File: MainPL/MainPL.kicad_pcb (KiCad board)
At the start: 2 copper layers, 113 x 155.6 mm, 37 parts, among them J1 Conn_01x06_Female, J10 Conn_01x06_Female, J11 Conn_01x06_Female, J12 Conn_01x06_Female, J13 Conn_01x06_Female, J14 Conn_01x06_Female, J15 Conn_01x01_Male, J16 Conn_01x04_Male, J2 USB_B, J3 Conn_01x06_Female, J4 Conn_01x06_Female, J5 Conn_01x06_Female, J6 Conn_01x06_Female, J7 Conn_01x09_Male, J8 Conn_01x06_Female, J9 Conn_01x06_Female, SW1 SW_Push_Dual, U1 74LS32, U2 ATmega328P-PU, U3 MCP23017_SP, U5 MCP23017_SP, U6 74LS373, U7 MCP23017_SP, U8 MC74HC589A, U9 74LVC2G04, Y1 Crystal_GND2

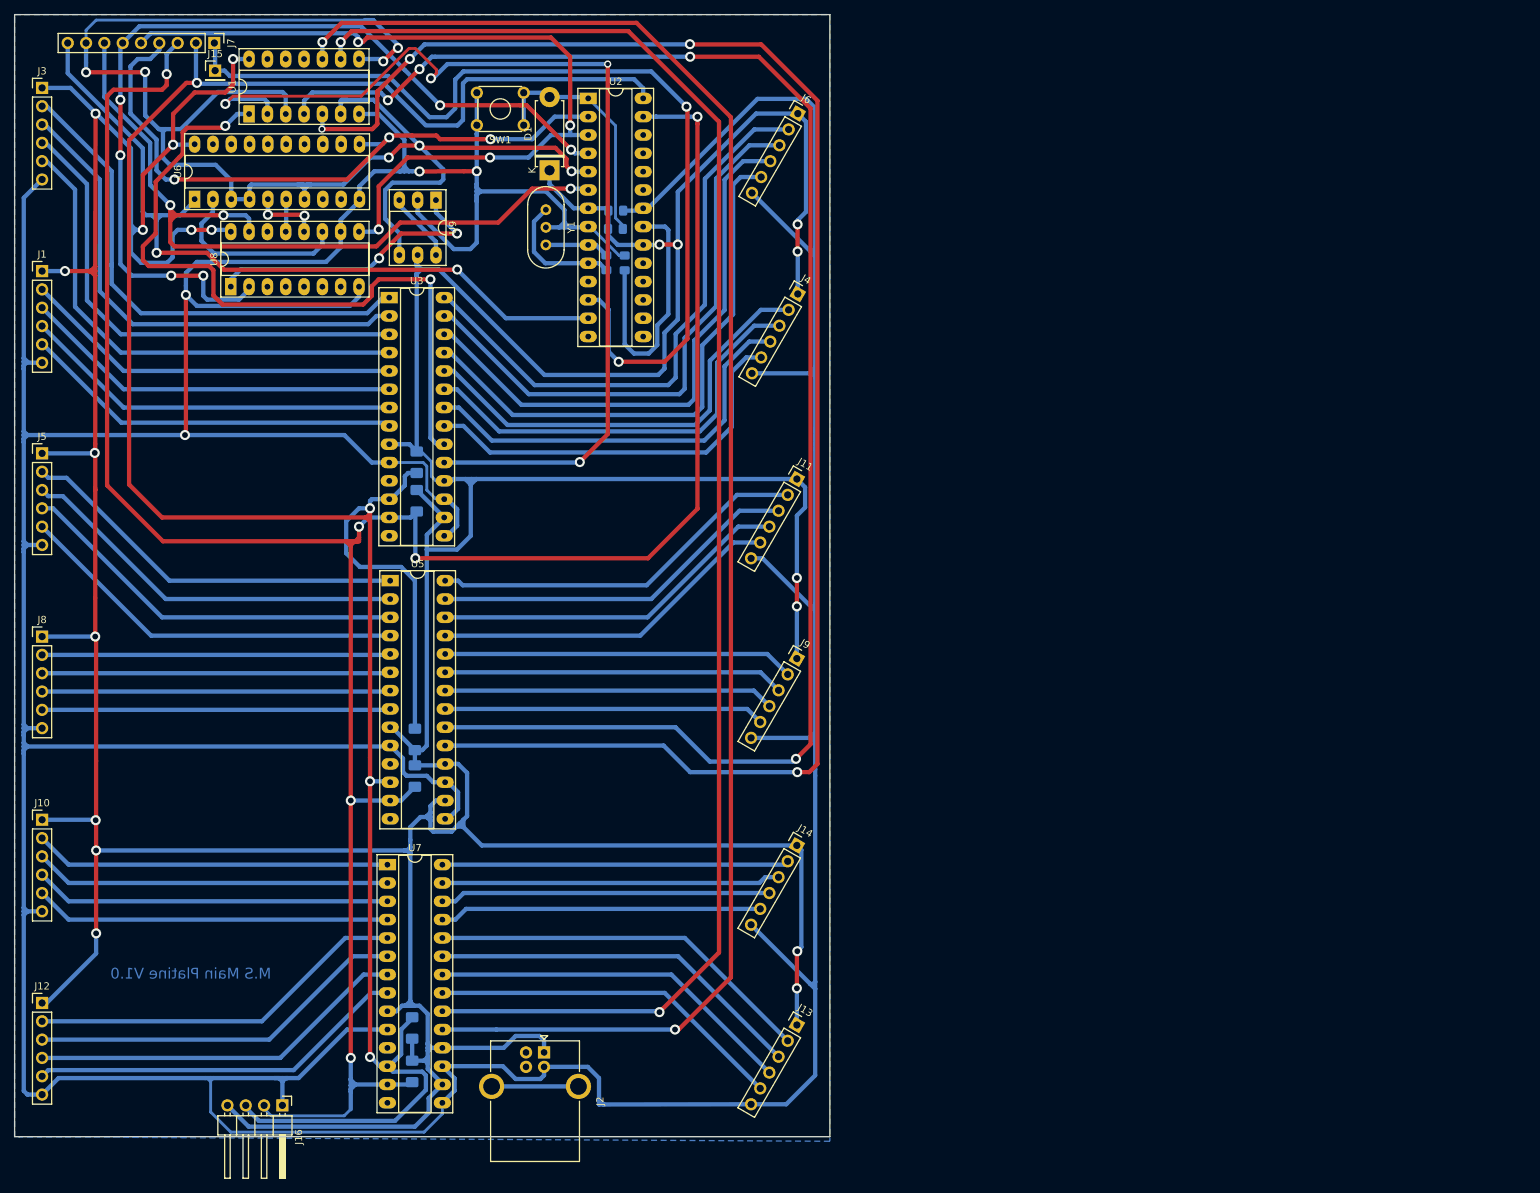
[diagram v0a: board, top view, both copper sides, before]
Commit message: Add files via upload
V.2 von Parkplatz mit neuen Maßen
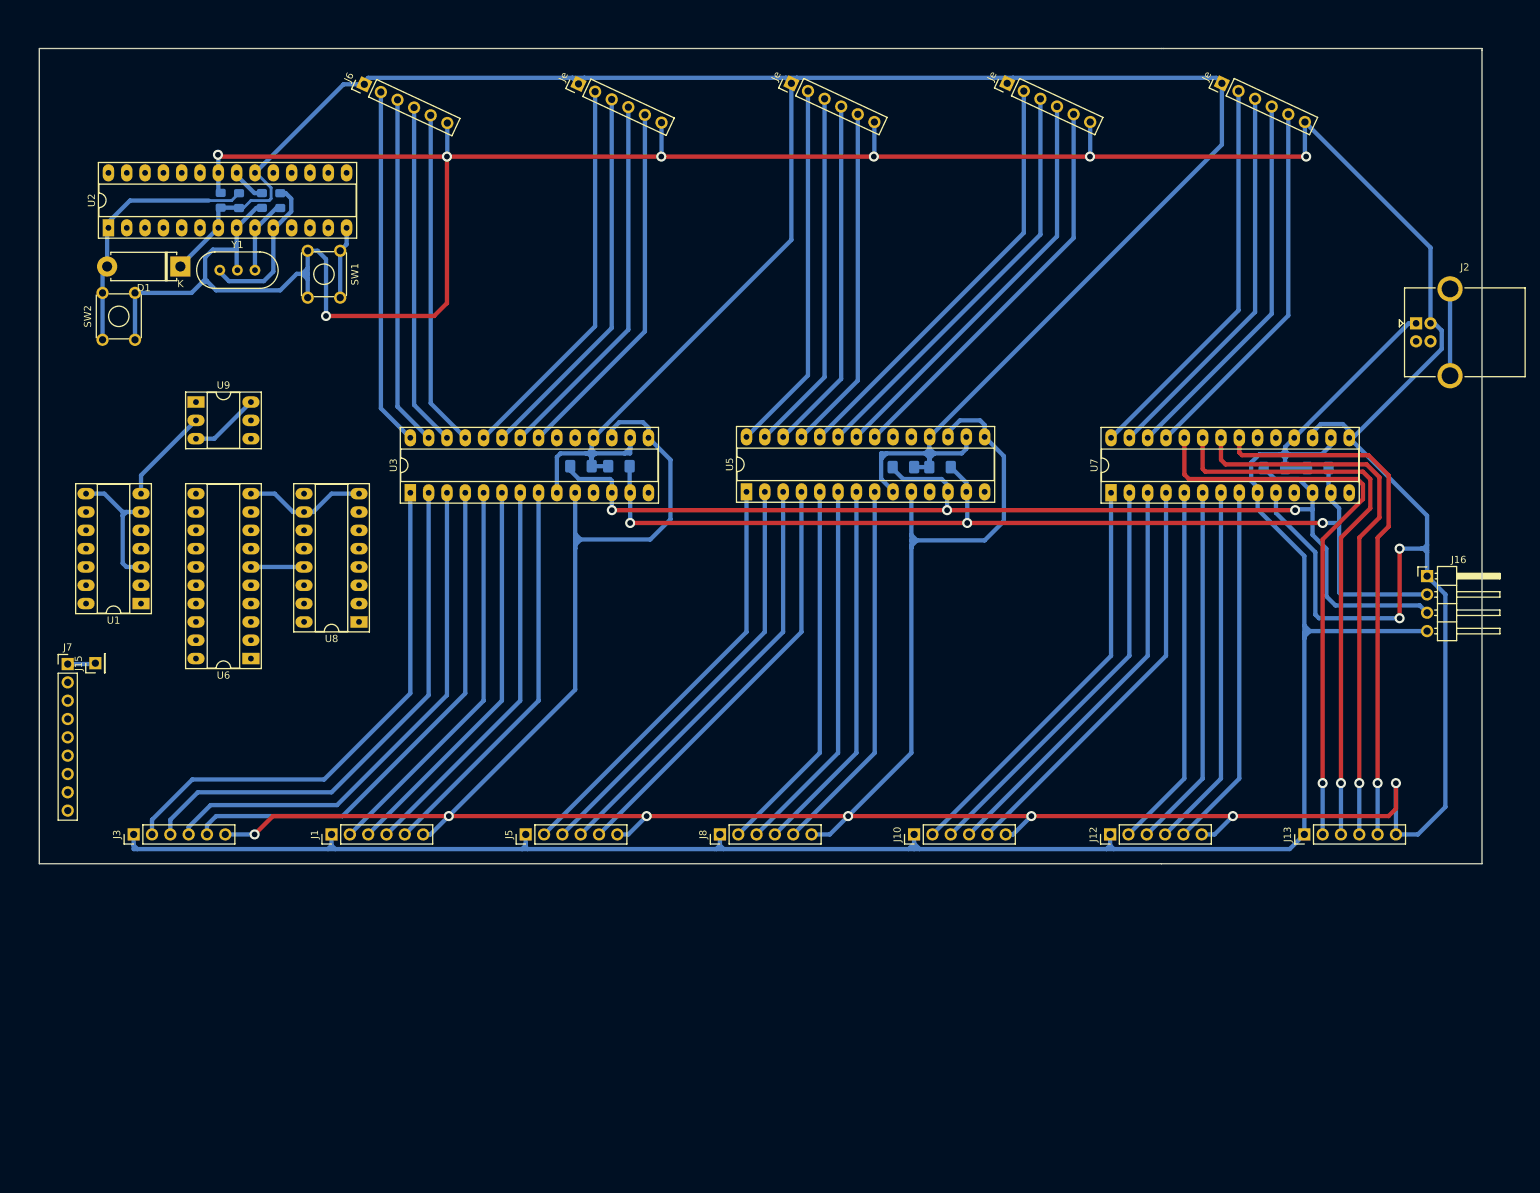
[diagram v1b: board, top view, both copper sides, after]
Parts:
- removed J14, J4, J9: Conn_01x06_Female, Connector_PinHeader_2.54mm:PinHeader_1x06_P2.54mm_Vertical
- added Je: Conn_01x06_Female, Connector_PinHeader_2.54mm:PinHeader_1x06_P2.54mm_Vertical, F.Cu at (122.6, 35.6)
- added Je: Conn_01x06_Female, Connector_PinHeader_2.54mm:PinHeader_1x06_P2.54mm_Vertical, F.Cu at (182.1, 35.6)
- added Je: Conn_01x06_Female, Connector_PinHeader_2.54mm:PinHeader_1x06_P2.54mm_Vertical, F.Cu at (211.8, 35.6)
- added SW2: SW_Push_MS, Button_Switch_THT:SW_TH_Tactile_Omron_B3F-10xx, F.Cu at (56.6, 71.1)
- SW1: value SW_Push_Dual -> SW_Push_MS
- moved J16 174.8 mm to (240.3, 103.9), turned to 0 degrees
- moved J2 157.6 mm to (238.8, 68.8), turned to 0 degrees
- moved R6 150.9 mm to (225.1, 88.9), turned to 0 degrees
- moved J12 149.9 mm to (196.3, 139.7), turned to 90 degrees
- moved R8 142.5 mm to (219.1, 88.9), turned to 0 degrees
- moved J10 120.9 mm to (169.2, 139.7), turned to 90 degrees
- moved U7 112.8 mm to (196.5, 92.3), turned to 90 degrees
- moved J3 104.3 mm to (61.0, 139.7), turned to 90 degrees
- moved J8 97.9 mm to (142.2, 139.7), turned to 90 degrees
- moved J7 88.5 mm to (51.8, 116.1), turned to 0 degrees
- moved J1 87.8 mm to (88.4, 139.7), turned to 90 degrees
- moved J5 85.4 mm to (115.3, 139.7), turned to 90 degrees
- moved R3 84.5 mm to (172.8, 88.8), turned to 0 degrees
- moved J15 83.8 mm to (55.6, 116.0), turned to 90 degrees
- moved R4 77.5 mm to (167.7, 88.8), turned to 0 degrees
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- renumbered J11 to Je
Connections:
- net /INTB_2 renamed Net-(U1-Pad5)
- SW1 pad 1: Net-(D1-Pad2) -> Net-(SW1-Pad1)
- SW1 pad 2: GND -> Net-(SW1-Pad1)
- SW1 pad 3: Net-(D1-Pad2) -> GND
- U2 pad 14: Net-(U2-Pad14) -> Net-(SW1-Pad1)
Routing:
- net Net-(U1-Pad10): track 227.8 -> 0.00 mm, vias 2 -> 0
- net Net-(U1-Pad5): track 227.4 -> 0.00 mm, vias 4 -> 0
- net Net-(U1-Pad4): track 220.3 -> 0.00 mm, vias 4 -> 0
- net Net-(U1-Pad9): track 217.7 -> 0.00 mm, vias 2 -> 0
- net /SDA: track 345.7 -> 145.1 mm, vias 6 -> 3
- net /INTArduino: track 218.0 -> 19.3 mm, vias 7 -> 0
- net /SCL: track 350.5 -> 158.8 mm, vias 4 -> 3
- net +5V: track 821.1 -> 661.1 mm, vias 20 -> 0
- net Net-(U1-Pad2): track 144.1 -> 0.00 mm, vias 4 -> 0
- net Servo: track 133.2 -> 3.88 mm, vias 2 -> 0
- net /CLK: track 126.1 -> 0.00 mm, vias 6 -> 0
- net /Qh: track 114.1 -> 0.00 mm, vias 4 -> 0
- net /CLK_INH: track 108.7 -> 0.00 mm, vias 3 -> 0
- net /OE: track 106.8 -> 0.00 mm, vias 2 -> 0
- net Net-(U1-Pad1): track 102.1 -> 0.00 mm, vias 2 -> 0
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- removed copper zone on B.Cu, net GND
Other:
- board size 113 x 155.6 mm -> 200 x 113 mm
- rule trace_min: 0.6 -> 0.4
- board text removed: "M.S Main Platine V1.0"
